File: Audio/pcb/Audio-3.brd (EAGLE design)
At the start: 41.9 x 17.8 mm, 61 parts, among them IC1 AUDIO-DAC-AMP-NXP-TFA988X, IC2 AUDIO-DAC-AMP-NXP-TFA988X, IC3 DRIVER-RS485-RS422-SN75176-SO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, IC4 LPC13XXFHN33, IC5 LDO-REGULATOR-FIXED-WITH-ENAB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, IC6 LDO-REGULATOR-FIXED-WITH-ENAB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, IC7 SWITCHING-REGULATOR-VARIABLE-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, K1 HEADER-1X02-0.1IN-NO-SILK, K2 HEADER-1X02-0.1IN-NO-SILK, K3 HEADER-1X02-0.1IN-NO-SILK, K4 HEADER-1X02-0.1IN-NO-SILK, K5 HEADER-1X02-0.1IN-NO-SILK, U4 GND-ISOLATOR-0.032", X1 CRYSTAL-4-PIN-NDK-NX3225GA-MIN

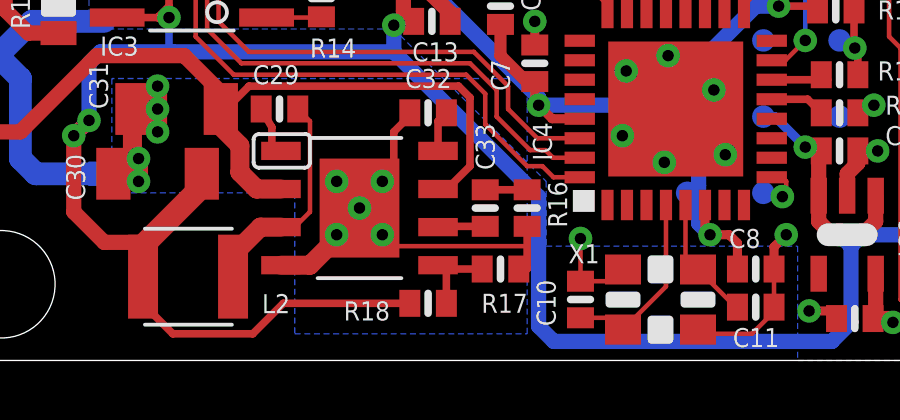
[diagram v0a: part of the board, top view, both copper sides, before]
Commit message: Updates to ambient audio etc.
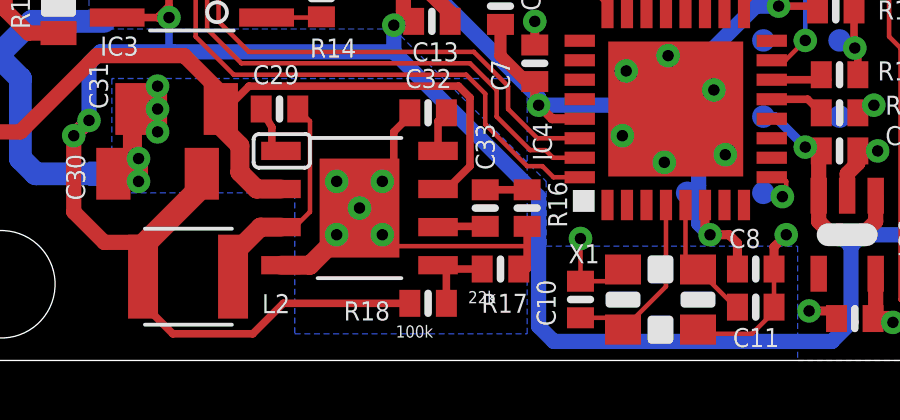
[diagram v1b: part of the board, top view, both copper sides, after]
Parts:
- R17: value (none) -> 22k
- R18: value (none) -> 100k
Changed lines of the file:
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@@
 <layer number="21" name="tPlace" color="7" fill="1" visible="yes" active="yes"/>
 <layer number="22" name="bPlace" color="7" fill="1" visible="yes" active="yes"/>
-<layer number="23" name="tOrigins" color="15" fill="1" visible="no" active="yes"/>
+<layer number="23" name="tOrigins" color="15" fill="1" visible="yes" active="yes"/>
 <layer number="24" name="bOrigins" color="15" fill="1" visible="no" active="yes"/>
 <layer number="25" name="tNames" color="7" fill="1" visible="no" active="yes"/>
@@
 <attribute name="VALUE" x="20.066" y="11.43" size="0.762" layer="37" font="vector" ratio="15" rot="R270"/>
 </element>
-<element name="R17" library="Outbreak" package="0603-MIN" value="" x="19.177" y="3.048" smashed="yes">
+<element name="R17" library="Outbreak" package="0603-MIN" value="22k" x="19.177" y="3.048" smashed="yes">
 <attribute name="NAME" x="18.542" y="1.5875" size="0.635" layer="21" font="vector" ratio="15"/>
 <attribute name="VALUE" x="18.0975" y="1.905" size="0.4064" layer="21" font="vector" ratio="10"/>
@@
 <attribute name="VALUE" x="12.827" y="3.048" size="0.762" layer="37" font="vector" ratio="15"/>
 </element>
-<element name="R18" library="Outbreak" package="0603-MIN" value="" x="16.764" y="1.905" smashed="yes">
+<element name="R18" library="Outbreak" package="0603-MIN" value="100k" x="16.764" y="1.905" smashed="yes">
 <attribute name="NAME" x="15.494" y="1.9685" size="0.635" layer="21" font="vector" ratio="15" rot="R180"/>
 <attribute name="VALUE" x="15.6845" y="0.762" size="0.4064" layer="21" font="vector" ratio="10"/>
